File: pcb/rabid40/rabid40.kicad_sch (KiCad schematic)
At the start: 12 parts

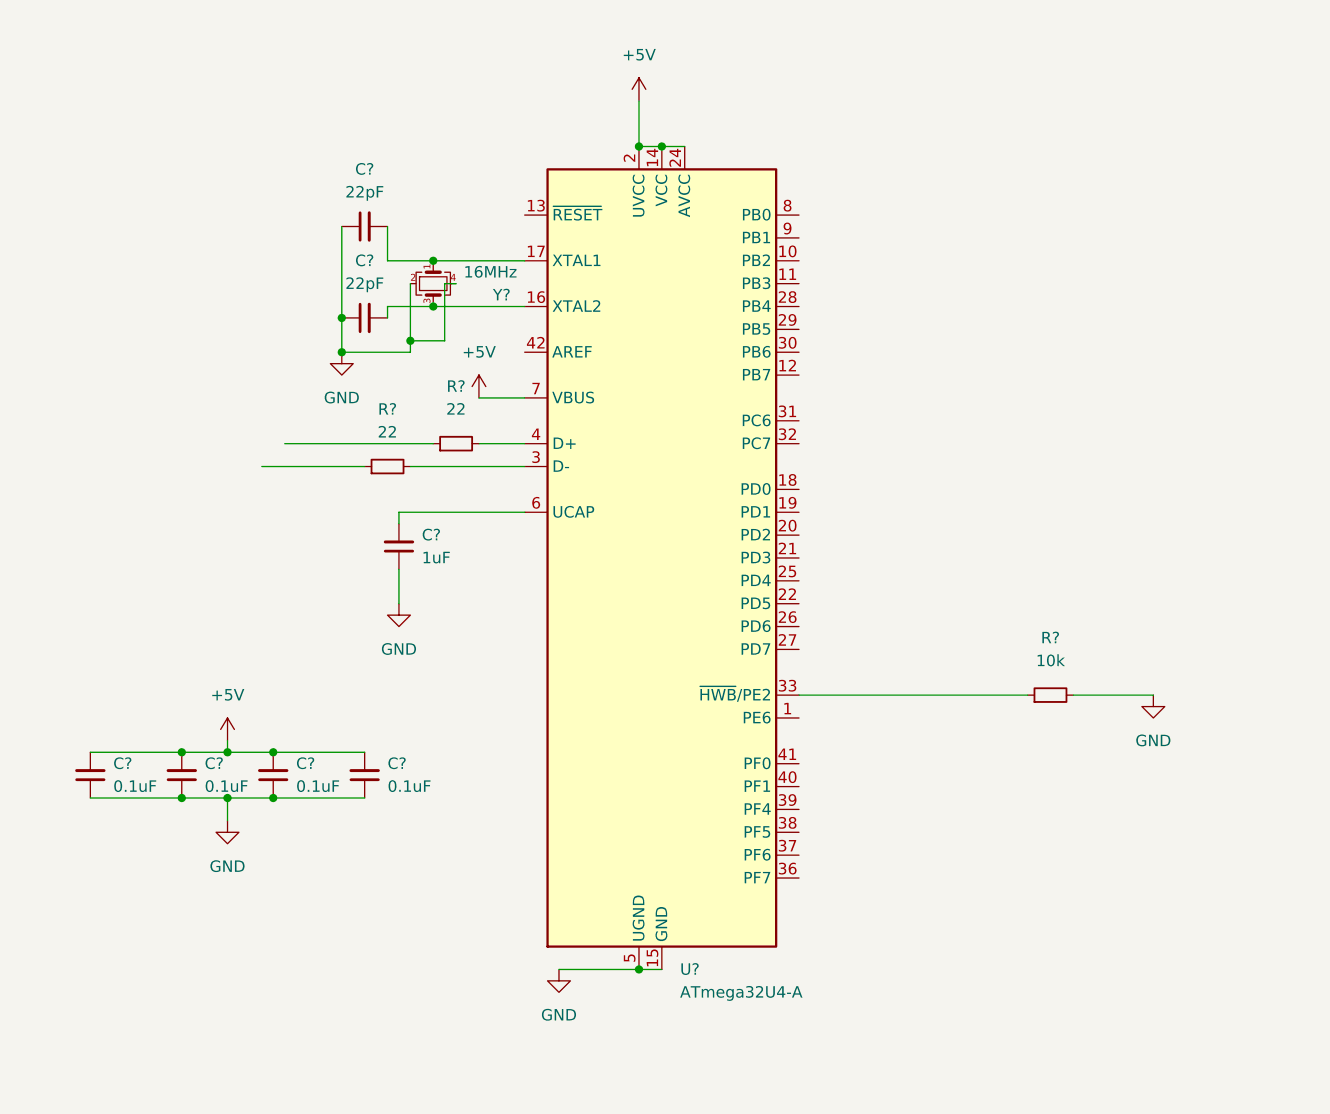
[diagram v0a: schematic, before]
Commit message: schematic basics laid down
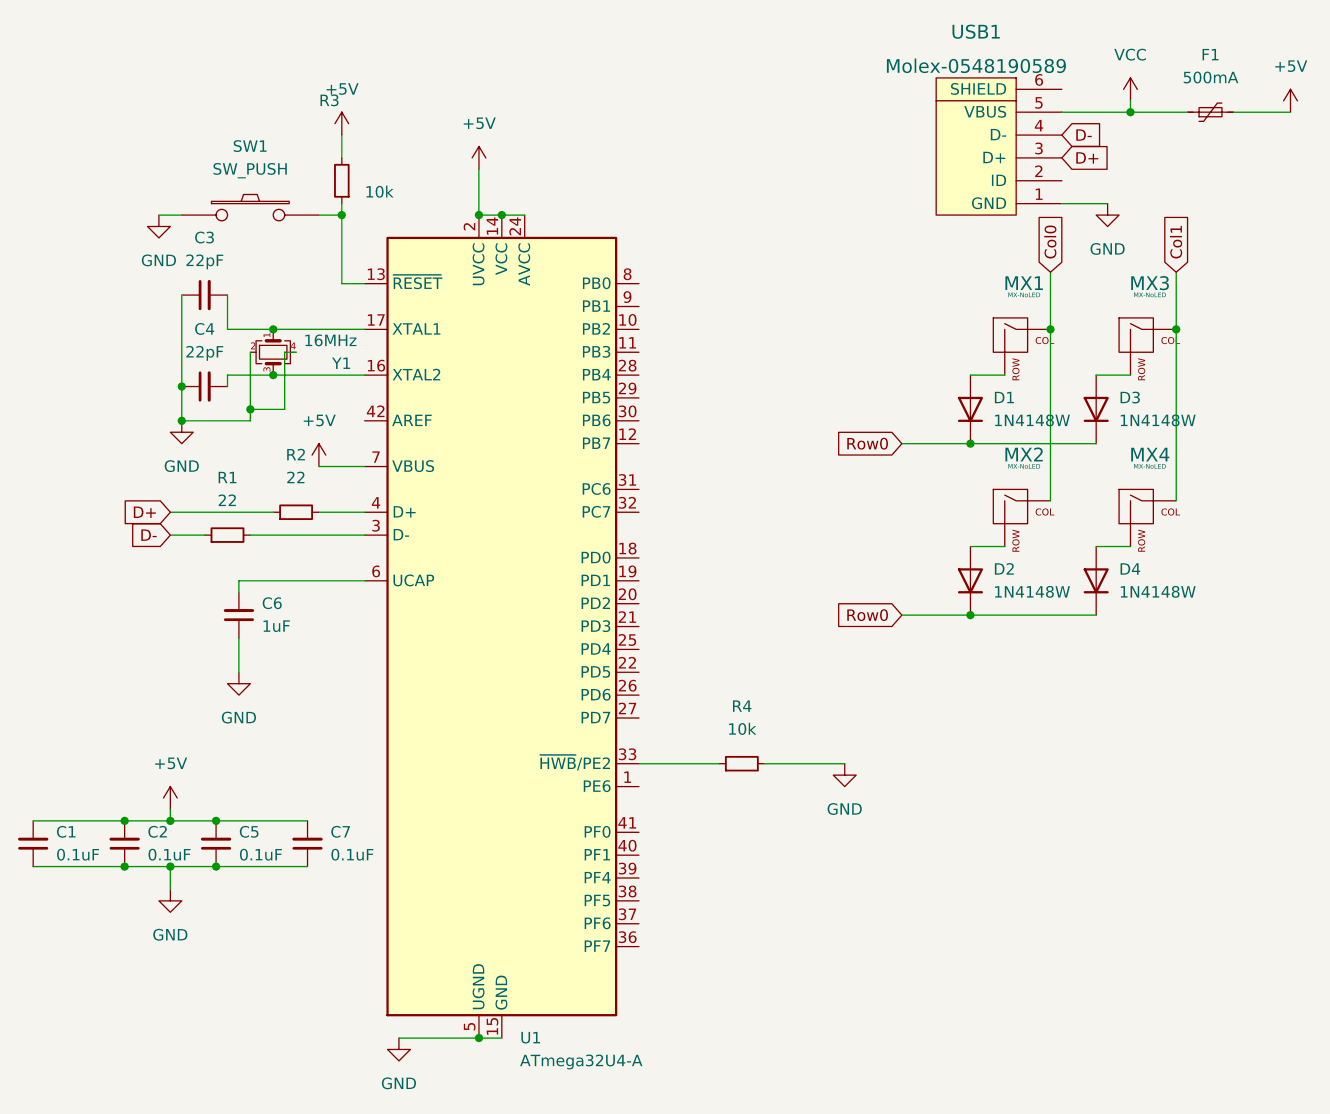
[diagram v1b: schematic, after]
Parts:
- added D1, D2, D3, D4: 1N4148W, Diode_SMD:D_SOD-123, symbol Diode:1N4148W
- added F1: 500mA, Fuse:Fuse_1206_3216Metric, symbol Device:Polyfuse_Small
- added MX1, MX2, MX3, MX4: MX-NoLED, MX_Alps_Hybrid:MX-1U-NoLED, symbol ai03-mx-alps-hybrid:MX-NoLED
- added R3: 10k, Resistor_SMD:R_0805_2012Metric, symbol Device:R_Small
- added SW1: SW_PUSH, random-keyboard-parts:SKQG-1155865, symbol Keyboard_Symbols:SW_PUSH
- added USB1: Molex-0548190589, random-keyboard-parts:Molex-0548190589, symbol ai03-random-parts:Molex-0548190589
- C1, C2, C3, C4, C5, C6, C7: renamed from C?; footprint (none) -> Capacitor_SMD:C_0805_2012Metric
- R1, R2, R4: renamed from R?; footprint (none) -> Resistor_SMD:R_0805_2012Metric
- Y1: renamed from Y?; footprint (none) -> Crystal:Crystal_SMD_3225-4Pin_3.2x2.5mm
- gave numbers to parts that had none: 1
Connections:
- net +5V: now also F1.2, R3.2
- net GND: now also SW1.1, USB1.1 (GND)
- net D+: now reaches R2.1
- net D+: now also USB1.3 (D+)
- net at U1.13 (~{RESET}): now also R3.1, SW1.2
- net D-: now reaches R1.1
- net D-: now also USB1.4 (D-)
- new net: D2.2 (A), MX2.2 (ROW)
- new net: D4.2 (A), MX4.2 (ROW)
- new net: D1.2 (A), MX1.2 (ROW)
- new net: D3.2 (A), MX3.2 (ROW)
- new net Col0: MX1.1 (COL), MX2.1 (COL)
- new net Col1: MX3.1 (COL), MX4.1 (COL)
- new net Row0: D1.1 (K), D2.1 (K), D3.1 (K), D4.1 (K)
- new net VCC: F1.1, USB1.5 (VBUS)
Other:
- moved on the sheet: C1, C2, C3, C4, C5, C6, C7, R1, R2, R4, U1, Y1
